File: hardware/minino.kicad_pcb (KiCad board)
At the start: 2 copper layers, 45 x 68 mm, 58 parts, among them J1 OLED, J2 GPS, J3 Battery, P1 USB_C_Plug_USB2.0, Q1 DMG3415U-7, Q2 PN2222A, SW1 ON, SW2 RIGHT, SW3 LEFT, SW4 DOWN, SW5 UP, SW6 OK, SW7 RESET, SW8 GPIO, U1 ESP32-S3-WROOM-1U-N16, U2 MCP73831-3-OT, U3 AP2112K-3.3

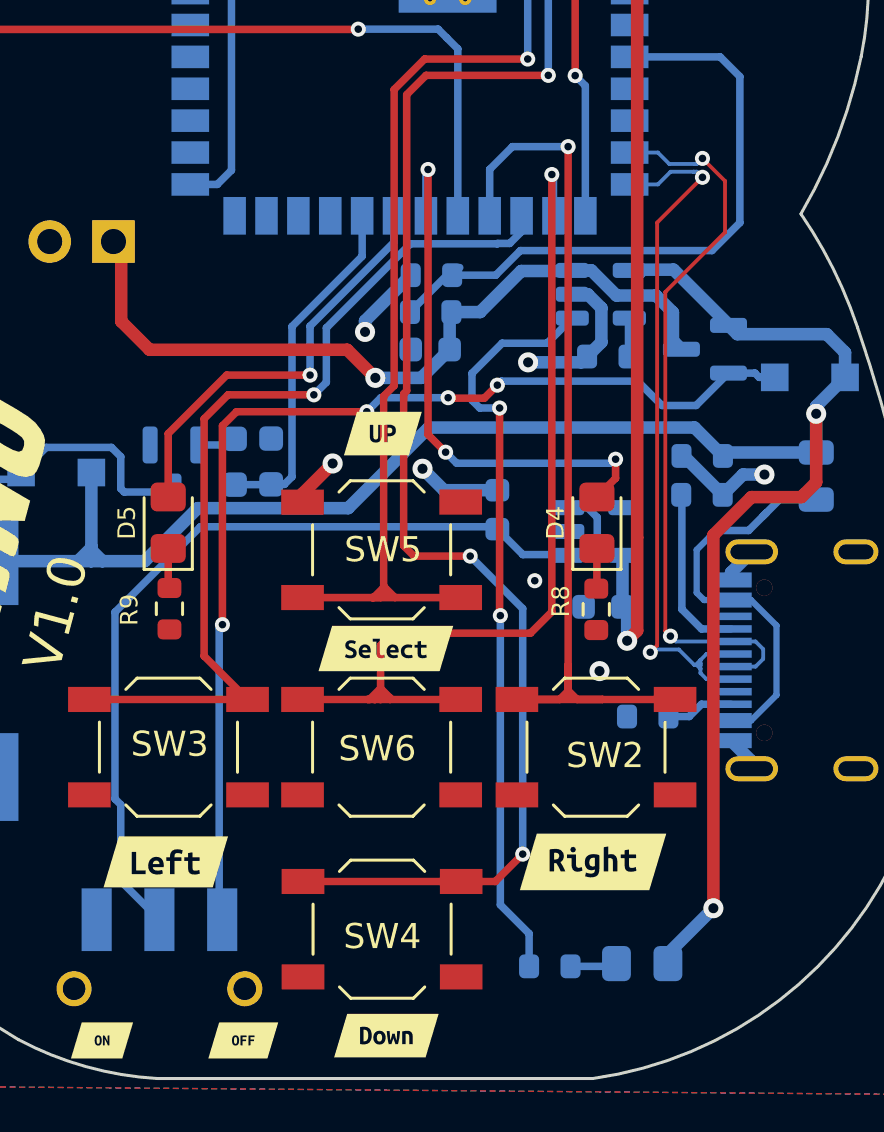
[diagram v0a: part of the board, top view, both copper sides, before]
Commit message: update usb
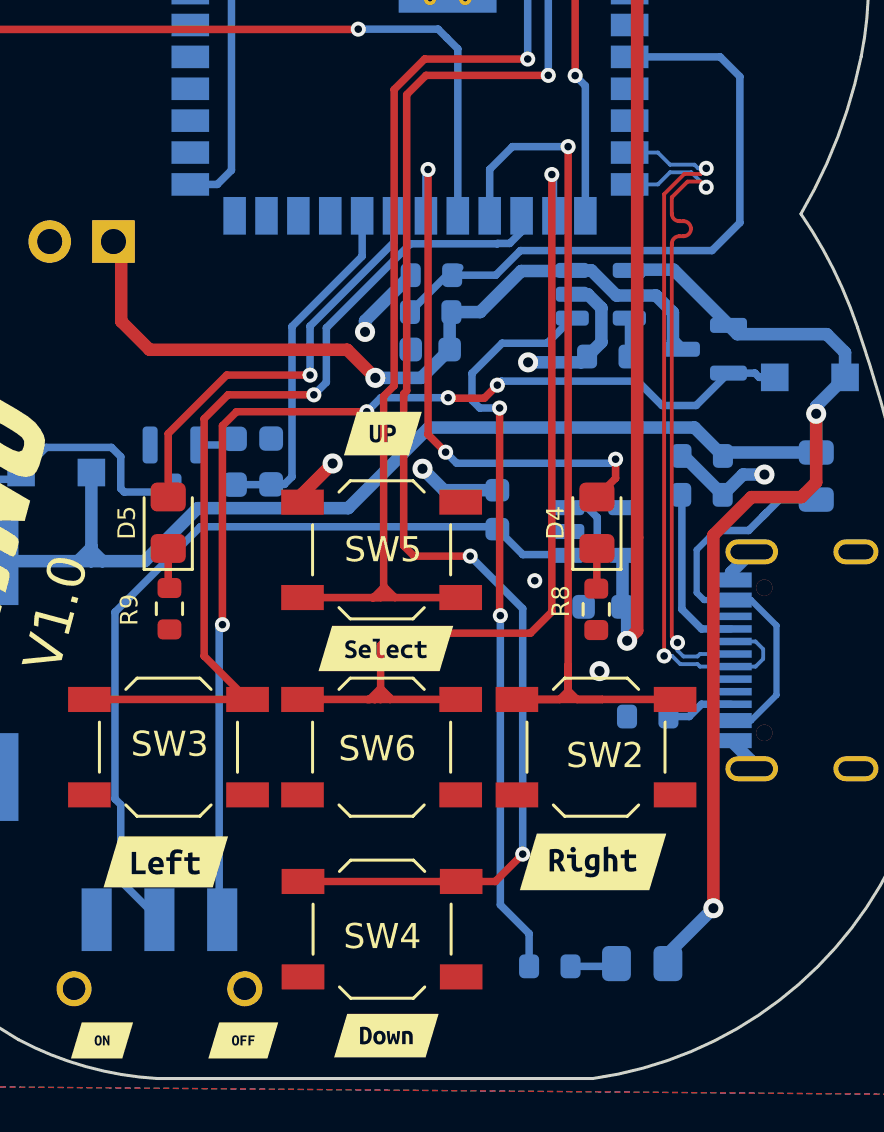
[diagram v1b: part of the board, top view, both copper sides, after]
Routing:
- net /D+: track 29.2 -> 26.6 mm
